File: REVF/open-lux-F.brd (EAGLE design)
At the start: 54.4 x 61.1 mm, 54 parts, among them IC2 MCP73831, IC3 ATMEGA32U4-AU, IC4 MCP1700-33, J1 AYZ0202, Q4 BSS123, T1 FDN340P, T2 FDN340P, X2 USBSMD, X3 8MHz

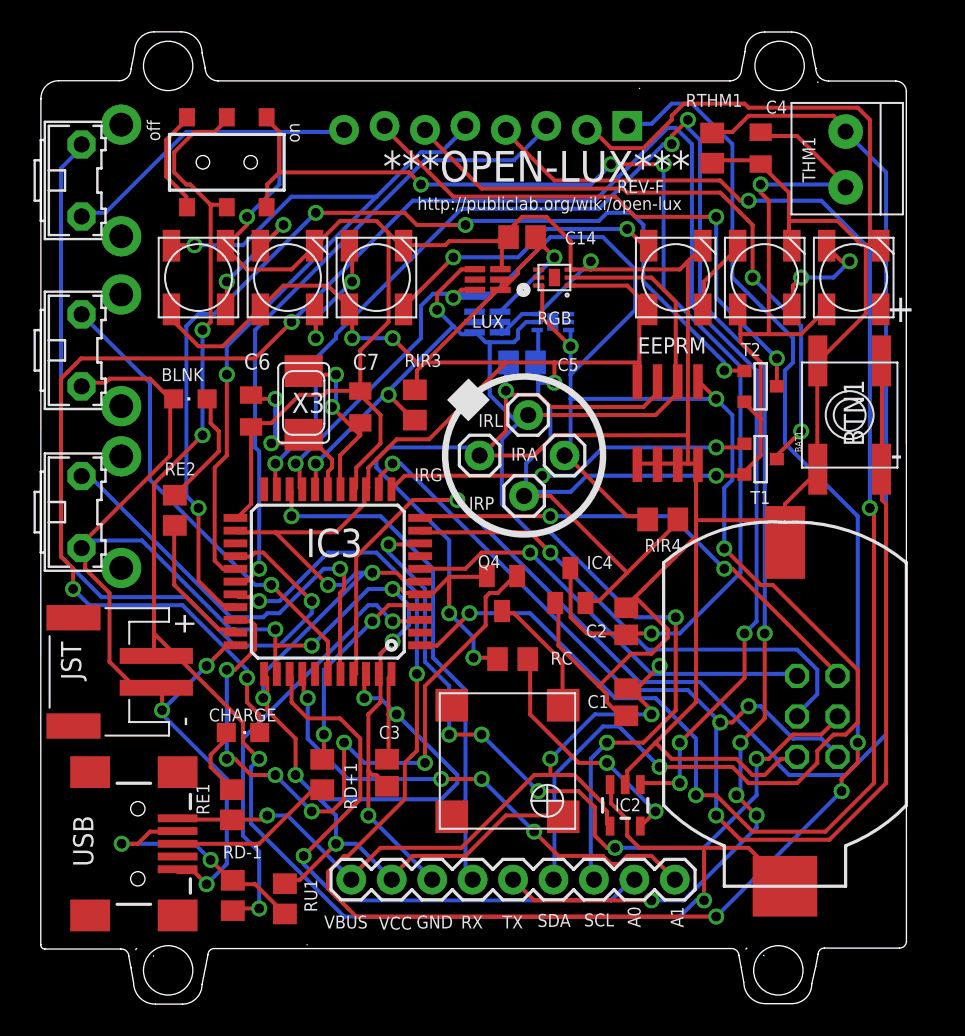
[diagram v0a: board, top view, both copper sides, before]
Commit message: update
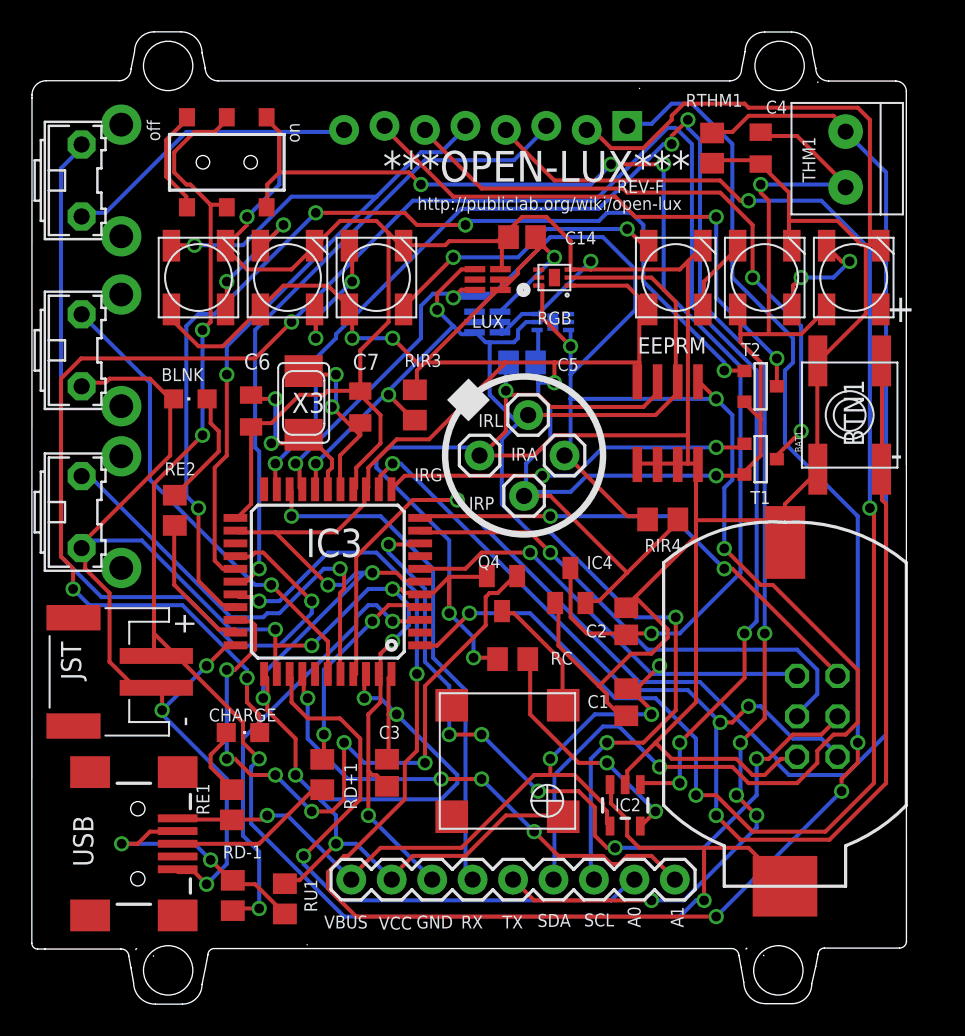
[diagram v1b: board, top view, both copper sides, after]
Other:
- board size 54.4 x 61.1 mm -> 54.9 x 61.1 mm
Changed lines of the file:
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@@
 <setting verticaltext="up"/>
 </settings>
-<grid distance="0.000393700787" unitdist="inch" unit="inch" style="lines" multiple="1" display="no" altdistance="0.025" altunitdist="inch" altunit="inch"/>
+<grid distance="0.393700787" unitdist="mil" unit="mil" style="lines" multiple="1" display="no" altdistance="0.025" altunitdist="inch" altunit="inch"/>
 <layers>
 <layer number="1" name="Top" color="4" fill="1" visible="yes" active="yes"/>
@@
 <text x="7.496" y="50.476" size="0.8128" layer="21" font="vector" rot="R90">off</text>
 <wire x1="54.356" y1="53.594" x2="54.366" y2="0.21" width="0" layer="20"/>
-<wire x1="0" y1="0" x2="0" y2="0.02" width="0" layer="20"/>
-<wire x1="0" y1="0.02" x2="0.01" y2="53.11" width="0" layer="20"/>
+<wire x1="-0.56" y1="0.1" x2="-0.55" y2="53.19" width="0" layer="20"/>
 <wire x1="7.07" y1="-0.69" x2="7.09" y2="-0.71" width="0" layer="20" curve="-90"/>
 <wire x1="16.72" y1="0.01" x2="16.73" y2="0" width="0" layer="20" curve="-90"/>
@@
 <wire x1="8.82" y1="57.34" x2="10.13" y2="56.01" width="0" layer="20" curve="-90"/>
 <wire x1="10.13" y1="56.01" x2="10.33" y2="55.06" width="0" layer="20"/>
-<wire x1="4.93" y1="54.27" x2="1.12" y2="54.27" width="0" layer="20"/>
-<wire x1="1.12" y1="54.27" x2="0.01" y2="53.16" width="0" layer="20" curve="90"/>
-<wire x1="0.01" y1="53.16" x2="0.01" y2="53.11" width="0" layer="20"/>
+<wire x1="4.93" y1="54.27" x2="0.34" y2="54.27" width="0" layer="20"/>
 <wire x1="10.33" y1="55.06" x2="10.33" y2="55.07" width="0" layer="20"/>
 <wire x1="10.33" y1="55.07" x2="11.14" y2="54.26" width="0" layer="20" curve="90"/>
@@
 <wire x1="6.03" y1="-0.24" x2="5.97" y2="-0.3" width="0" layer="20" curve="90"/>
 <wire x1="5.53" y1="-0.7" x2="5.03" y2="-0.26" width="0" layer="20" curve="90"/>
-<wire x1="5.03" y1="-0.26" x2="0.26" y2="-0.26" width="0" layer="20"/>
-<wire x1="0.26" y1="-0.26" x2="0" y2="0" width="0" layer="20" curve="-90"/>
+<wire x1="5.03" y1="-0.26" x2="0.27" y2="-0.26" width="0" layer="20"/>
+<wire x1="0.27" y1="-0.26" x2="0.26" y2="-0.26" width="0" layer="20"/>
 <wire x1="45.39" y1="-0.66" x2="45.41" y2="-0.68" width="0" layer="20" curve="-90"/>
 <hole x="46.32" y="-1.6" drill="3.1"/>
@@
 <wire x1="49.21" y1="-0.2" x2="53.93" y2="-0.2" width="0" layer="20"/>
 <wire x1="53.93" y1="-0.2" x2="54.37" y2="0.24" width="0" layer="20" curve="90"/>
+<wire x1="-0.55" y1="53.19" x2="-0.55" y2="53.38" width="0" layer="20"/>
+<wire x1="0.34" y1="54.27" x2="-0.55" y2="53.38" width="0" layer="20" curve="90"/>
+<wire x1="0.26" y1="-0.26" x2="-0.2" y2="-0.26" width="0" layer="20"/>
+<wire x1="-0.2" y1="-0.26" x2="-0.56" y2="0.1" width="0" layer="20" curve="-90"/>
 </plain>
 <attributes>
@@
 </class>
 </classes>
-<designrules name="default">
+<designrules name="LaenPCBOrder">
 <description language="de">&lt;b&gt;EAGLE Design Rules&lt;/b&gt;
 &lt;p&gt;
@@
 Einstellungen hier und speichern die Design Rules unter
 einem neuen Namen ab.</description>
-<description language="en">&lt;b&gt;EAGLE Design Rules&lt;/b&gt;
+<description language="en">&lt;b&gt;Laen's PCB Order Design Rules&lt;/b&gt;
 &lt;p&gt;
-The default Design Rules have been set to cover
-a wide range of applications. Your particular design
-may have different requirements, so please make the
-necessary adjustments and save your customized
-design rules under a new name.</description>
+Please make sure your boards conform to these design rules.</description>
 <param name="layerSetup" value="(1*16)"/>
-<param name="mtCopper" value="0.035mm 0.035mm 0.035mm 0.035mm 0.035mm 0.035mm 0.035mm 0.035mm 0.035mm 0.035mm 0.035mm 0.035mm 0.035mm 0.035mm 0.035mm 0.035mm"/>
-<param name="mtIsolate" value="1.5mm 0.15mm 0.2mm 0.15mm 0.2mm 0.15mm 0.2mm 0.15mm 0.2mm 0.15mm 0.2mm 0.15mm 0.2mm 0.15mm 0.2mm"/>
-<param name="mdWireWire" value="8mil"/>
-<param name="mdWirePad" value="8mil"/>
-<param name="mdWireVia" value="8mil"/>
-<param name="mdPadPad" value="8mil"/>
-<param name="mdPadVia" value="8mil"/>
-<param name="mdViaVia" value="8mil"/>
-<param name="mdSmdPad" value="8mil"/>
-<param name="mdSmdVia" value="8mil"/>
-<param name="mdSmdSmd" value="8mil"/>
+<param name="mtCopper" value="0.0356mm 0.0356mm 0.0356mm 0.0356mm 0.0356mm 0.0356mm 0.0356mm 0.0356mm 0.0356mm 0.0356mm 0.0356mm 0.0356mm 0.0356mm 0.0356mm 0.0356mm 0.0356mm"/>
+<param name="mtIsolate" value="1.5011mm 0.1499mm 0.2007mm 0.1499mm 0.2007mm 0.1499mm 0.2007mm 0.1499mm 0.2007mm 0.1499mm 0.2007mm 0.1499mm 0.2007mm 0.1499mm 0.2007mm"/>
+<param name="mdWireWire" value="6mil"/>
+<param name="mdWirePad" value="6mil"/>
+<param name="mdWireVia" value="6mil"/>
+<param name="mdPadPad" value="6mil"/>
+<param name="mdPadVia" value="6mil"/>
+<param name="mdViaVia" value="6mil"/>
+<param name="mdSmdPad" value="6mil"/>
+<param name="mdSmdVia" value="6mil"/>
+<param name="mdSmdSmd" value="6mil"/>
 <param name="mdViaViaSameLayer" value="8mil"/>
 <param name="mnLayersViaInSmd" value="2"/>
-<param name="mdCopperDimension" value="40mil"/>
-<param name="mdDrill" value="8mil"/>
+<param name="mdCopperDimension" value="15mil"/>
+<param name="mdDrill" value="6mil"/>
 <param name="mdSmdStop" value="0mil"/>
-<param name="msWidth" value="10mil"/>
-<param name="msDrill" value="24mil"/>
-<param name="msMicroVia" value="9.99mm"/>
+<param name="msWidth" value="6mil"/>
+<param name="msDrill" value="13mil"/>
+<param name="msMicroVia" value="13mil"/>
 <param name="msBlindViaRatio" value="0.5"/>
 <param name="rvPadTop" value="0.25"/>
@@
 <param name="rvMicroViaOuter" value="0.25"/>
 <param name="rvMicroViaInner" value="0.25"/>
-<param name="rlMinPadTop" value="10mil"/>
+<param name="rlMinPadTop" value="7mil"/>
 <param name="rlMaxPadTop" value="20mil"/>
-<param name="rlMinPadInner" value="10mil"/>
+<param name="rlMinPadInner" value="7mil"/>
 <param name="rlMaxPadInner" value="20mil"/>
-<param name="rlMinPadBottom" value="10mil"/>
+<param name="rlMinPadBottom" value="7mil"/>
 <param name="rlMaxPadBottom" value="20mil"/>
-<param name="rlMinViaOuter" value="8mil"/>
+<param name="rlMinViaOuter" value="7mil"/>
 <param name="rlMaxViaOuter" value="20mil"/>
-<param name="rlMinViaInner" value="8mil"/>
+<param name="rlMinViaInner" value="7mil"/>
 <param name="rlMaxViaInner" value="20mil"/>
 <param name="rlMinMicroViaOuter" value="4mil"/>
@@
 <param name="mvStopFrame" value="1"/>
 <param name="mvCreamFrame" value="0"/>
-<param name="mlMinStopFrame" value="4mil"/>
-<param name="mlMaxStopFrame" value="4mil"/>
+<param name="mlMinStopFrame" value="3mil"/>
+<param name="mlMaxStopFrame" value="3mil"/>
 <param name="mlMinCreamFrame" value="0mil"/>
 <param name="mlMaxCreamFrame" value="0mil"/>
